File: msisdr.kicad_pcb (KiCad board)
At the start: 2 copper layers, 46.3 x 90.7 mm, 70 parts, among them J1 VCC_GPIO, J10 SMA_VHF1, J11 USB_OTG, J2 GPIO0, J3 GPIO1, J4 GPIO2, J5 GPIO3, J6 SMA_0_30MHZ, J7 SMA_30_60MHZ, J8 SMA_VHF2, J9 SMA_UHF, U1 msi2500, U2 msi001, U3 LP5900SDX-2.8, U4 AP7313-30SAG, Y1 24MHz

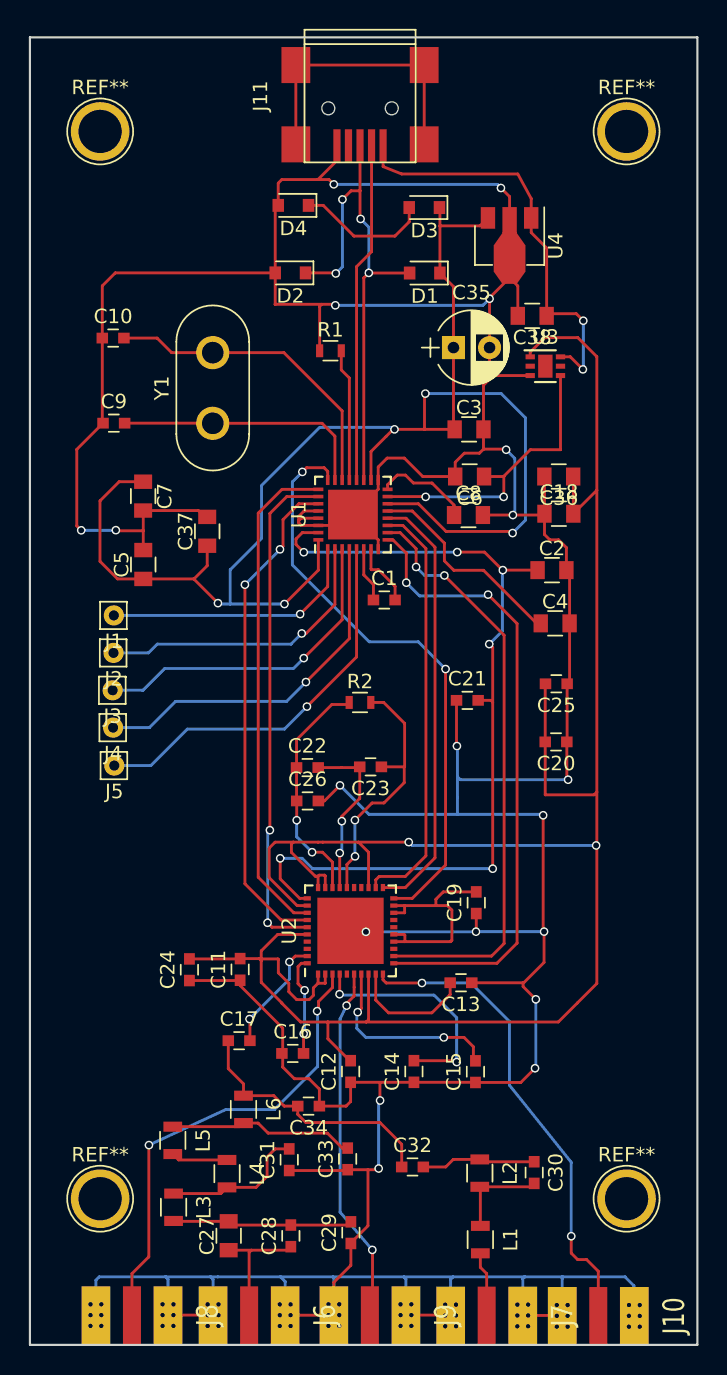
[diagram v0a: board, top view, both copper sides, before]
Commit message: finally version of pcb
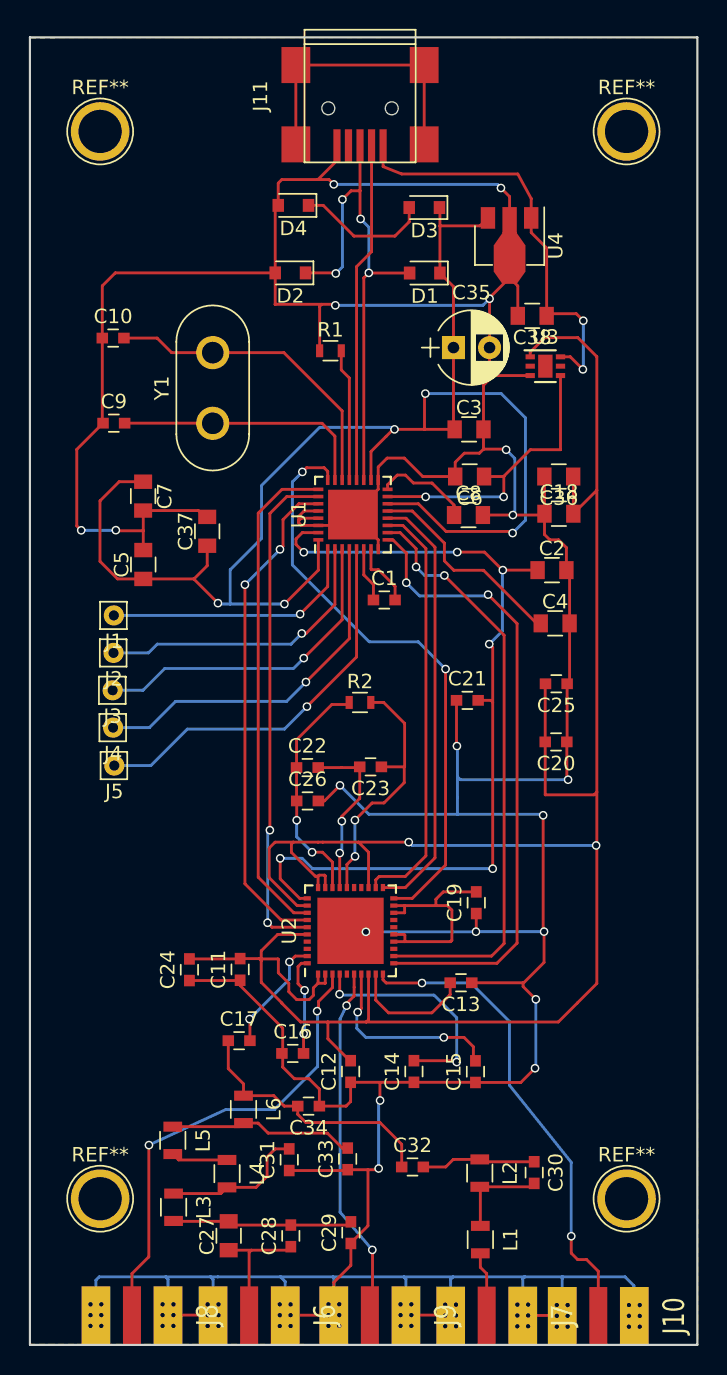
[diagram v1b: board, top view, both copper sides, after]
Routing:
- added copper zone on B.Cu, net GND
- added copper zone on F.Cu, net GND
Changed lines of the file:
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@@
   (general
     (links 234)
-    (no_connects 2)
-    (area 113.056599 42.470999 159.490481 144.007101)
+    (no_connects 0)
+    (area 99.214908 36.92012 159.490481 144.007101)
     (thickness 1.6)
-    (drawings 5)
+    (drawings 7)
     (tracks 823)
     (zones 0)
@@
   (layers
     (0 F.Cu signal)
-    (31 B.Cu signal)
+    (31 B.Cu signal hide)
     (32 B.Adhes user)
     (33 F.Adhes user)
@@
     (visible_elements 7FFEFFFF)
     (pcbplotparams
-      (layerselection 0x00030_80000001)
+      (layerselection 0x01fff_80000001)
       (usegerberextensions false)
       (excludeedgelayer true)
@@
       (outputformat 1)
       (mirror false)
-      (drillshape 1)
+      (drillshape 0)
       (scaleselection 1)
-      (outputdirectory ""))
+      (outputdirectory Gerber/))
   )
   (net 0 "")
@@
     )
   )
+  (dimension 90.600001 (width 0.3) (layer Eco2.User)
+    (gr_text "90.600 mm" (at 105.714907 88.809181 89.99367596) (layer Eco2.User)
+      (effects (font (size 1.5 1.5) (thickness 0.3)))
+    )
+    (feature1 (pts (xy 113.13 134.11) (xy 104.359907 134.109032)))
+    (feature2 (pts (xy 113.14 43.51) (xy 104.369907 43.509032)))
+    (crossbar (pts (xy 107.069907 43.50933) (xy 107.059907 134.10933)))
+    (arrow1a (pts (xy 107.059907 134.10933) (xy 106.473611 132.982762)))
+    (arrow1b (pts (xy 107.059907 134.10933) (xy 107.646452 132.982891)))
+    (arrow2a (pts (xy 107.069907 43.50933) (xy 106.483362 44.635769)))
+    (arrow2b (pts (xy 107.069907 43.50933) (xy 107.656203 44.635898)))
+  )
+  (dimension 46.27001 (width 0.3) (layer Eco2.User)
+    (gr_text "46.270 mm" (at 136.268378 38.285119 359.9628512) (layer Eco2.User)
+      (effects (font (size 1.5 1.5) (thickness 0.3)))
+    )
+    (feature1 (pts (xy 159.4 43.51) (xy 159.404254 36.95012)))
+    (feature2 (pts (xy 113.13 43.48) (xy 113.134254 36.92012)))
+    (crossbar (pts (xy 113.132503 39.620119) (xy 159.402503 39.650119)))
+    (arrow1a (pts (xy 159.402503 39.650119) (xy 158.275619 40.235809)))
+    (arrow1b (pts (xy 159.402503 39.650119) (xy 158.27638 39.062968)))
+    (arrow2a (pts (xy 113.132503 39.620119) (xy 114.258626 40.20727)))
+    (arrow2b (pts (xy 113.132503 39.620119) (xy 114.259387 39.034429)))
+  )
   (gr_line (start 159.41548 134.13232) (end 113.13668 134.13232) (angle 90) (layer Edge.Cuts) (width 0.15))
   (gr_line (start 113.1316 134.08914) (end 113.157 134.08914) (angle 90) (layer Edge.Cuts) (width 0.15))
@@
   (segment (start 121.3755 120.2903) (end 121.3755 128.0392) (width 0.2) (layer F.Cu) (net 26))
   (segment (start 134.109 108.426) (end 134.109 109.35762) (width 0.2) (layer F.Cu) (net 26))
-  (segment (start 120.2055 129.1945) (end 120.2055 132.0692) (width 0.2) (layer F.Cu) (net 26) (status 800000))
+  (segment (start 120.2055 129.1945) (end 120.2055 132.0692) (width 0.2) (layer F.Cu) (net 26))
   (segment (start 121.3608 128.0392) (end 120.2055 129.1945) (width 0.2) (layer F.Cu) (net 26))
   (segment (start 135.08736 110.61192) (end 135.08736 110.4646) (width 0.2) (layer F.Cu) (net 27))
@@
   (segment (start 135.08736 110.4646) (end 135.609 109.94296) (width 0.2) (layer F.Cu) (net 27))
   (segment (start 136.88568 131.88632) (end 136.7028 132.0692) (width 0.2) (layer F.Cu) (net 27))
-  (segment (start 152.5397 132.12254) (end 152.5397 129.0297) (width 0.2) (layer F.Cu) (net 28) (status 400000))
+  (segment (start 152.5397 132.12254) (end 152.5397 129.0297) (width 0.2) (layer F.Cu) (net 28))
   (segment (start 137.609 108.82064) (end 137.83056 109.0422) (width 0.2) (layer F.Cu) (net 28))
   (segment (start 137.83056 109.0422) (end 140.31468 109.0422) (width 0.2) (layer F.Cu) (net 28))
@@
   (segment (start 138.909 52.95) (end 146.959 52.95) (width 0.2) (layer F.Cu) (net 61))
   (segment (start 137.619 52.436) (end 138.909 52.95) (width 0.2) (layer F.Cu) (net 61))
+  (zone (net 35) (net_name GND) (layer F.Cu) (hatch edge 0.508)
+    (connect_pads (clearance 0.508))
+    (min_thickness 0.254)
+    (fill yes (arc_segments 16) (thermal_gap 0.508) (thermal_bridge_width 0.508))
+    (polygon
+      (pts
+        (xy 113.15 43.48) (xy 159.39 43.5) (xy 159.43 134.13) (xy 113.15 134.1)
+      )
+    )
+  )
+  (zone (net 35) (net_name GND) (layer B.Cu) (hatch edge 0.508)
+    (connect_pads (clearance 0.508))
+    (min_thickness 0.254)
+    (fill yes (arc_segments 16) (thermal_gap 0.508) (thermal_bridge_width 0.508))
+    (polygon
+      (pts
+        (xy 159.4 134.13) (xy 113.16 134.14) (xy 113.14 43.51) (xy 159.38 43.46)
+      )
+    )
+  )
 )
